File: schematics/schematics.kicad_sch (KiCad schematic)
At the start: 28 parts, among them SW1 RESET, U1 STM32F103VBT6, U2 AMS1117-3.3, Y1 16Mhz

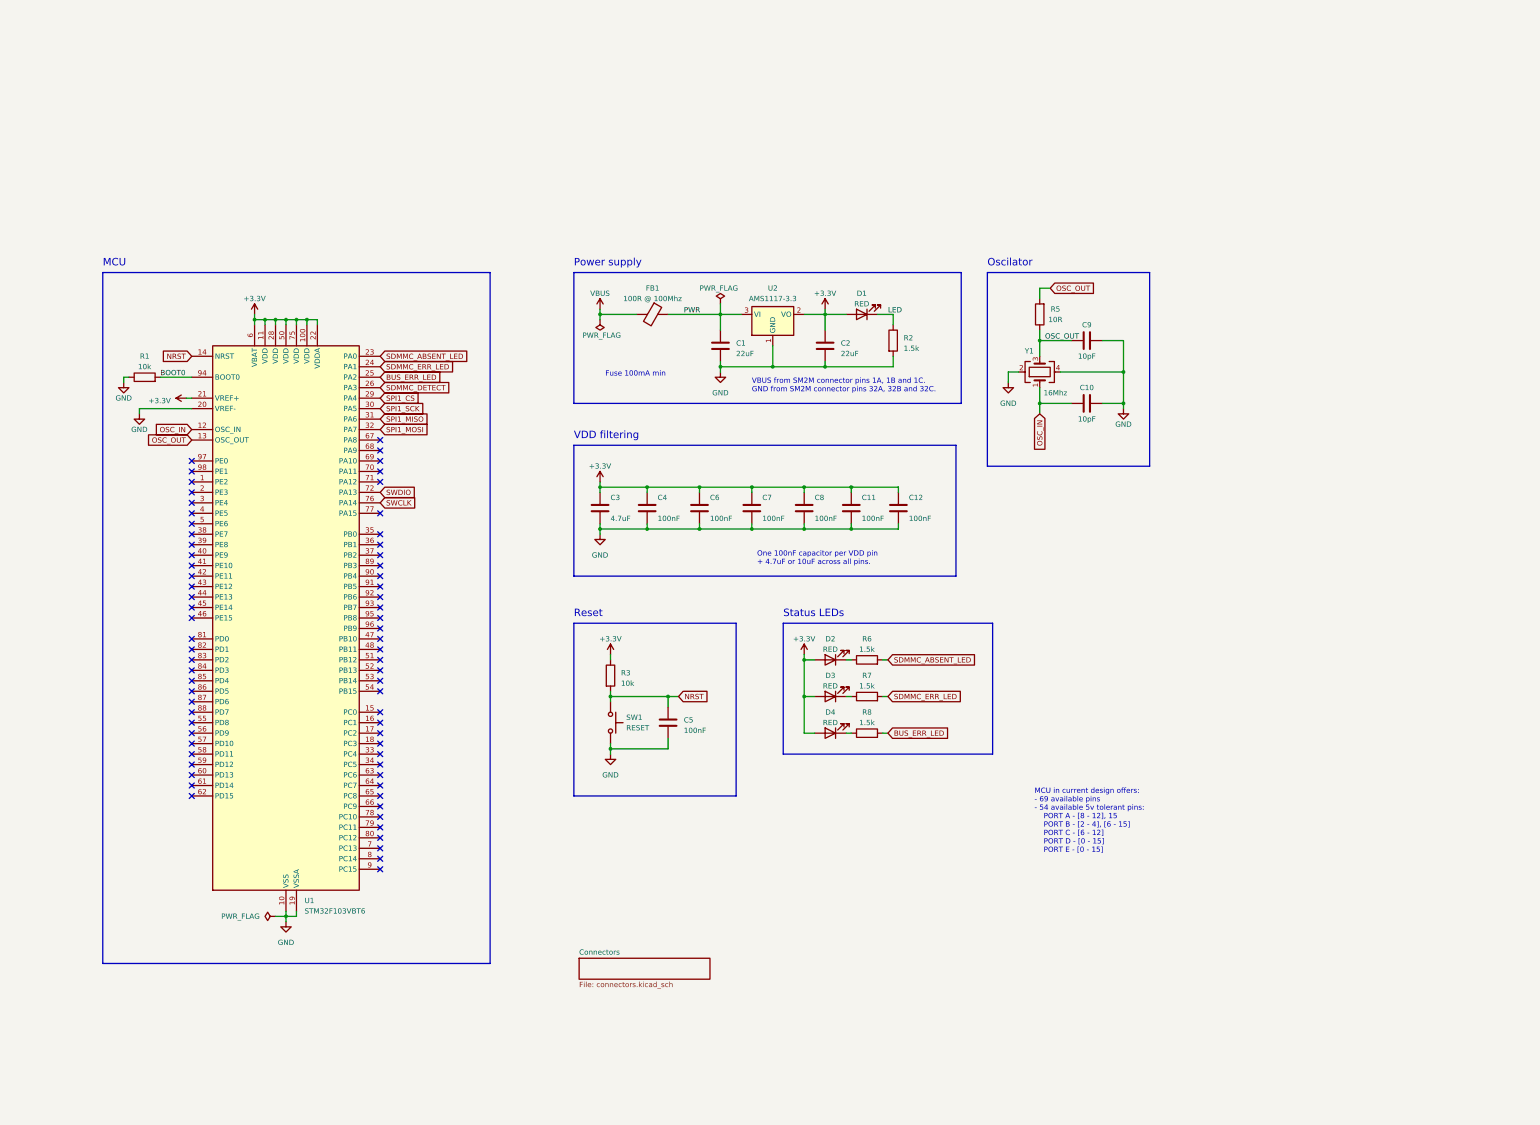
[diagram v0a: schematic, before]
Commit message: Update the board schematics
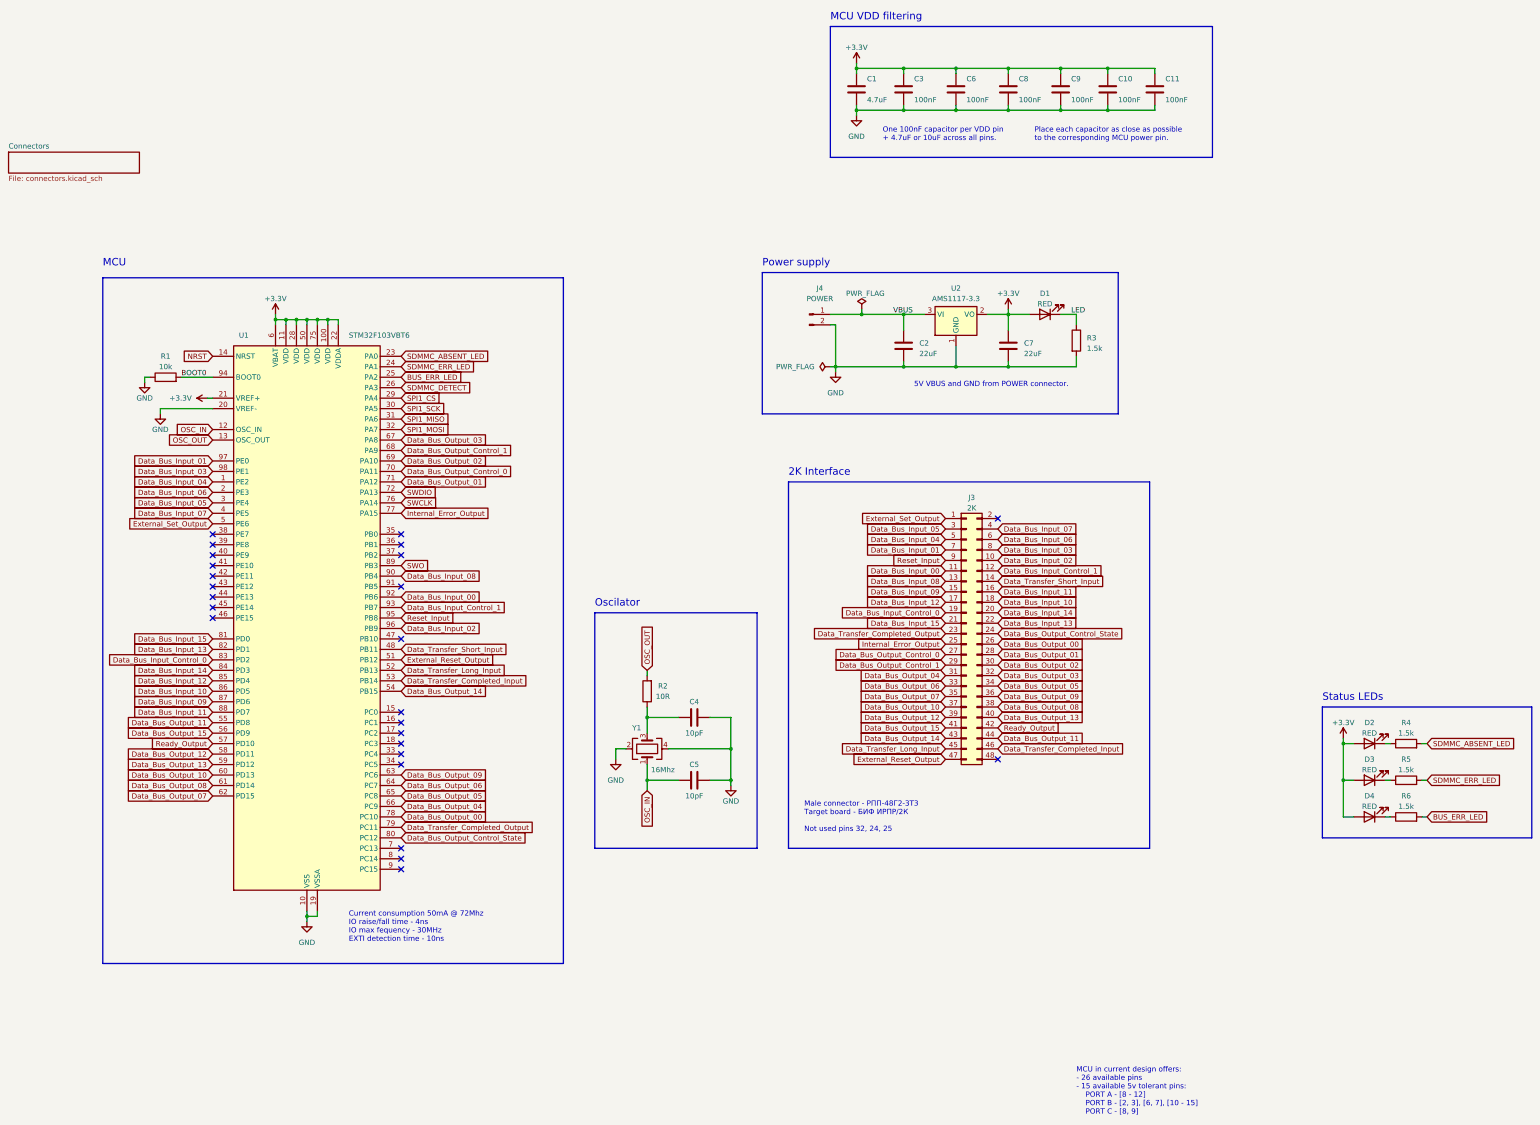
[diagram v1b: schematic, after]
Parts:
- removed C5: 100nF, Capacitor_SMD:C_0603_1608Metric, symbol Device:C
- removed FB1: 100R @ 100Mhz, Inductor_SMD:L_0603_1608Metric, symbol Device:FerriteBead
- removed R3: 10k, Resistor_SMD:R_0603_1608Metric, symbol Device:R
- removed SW1: RESET, Custom:SW_Push_SMD_4x4x1.5, symbol Switch:SW_Push
- added J3: 2K, Custom:RPP_48G2_3T3_Male, symbol Connector_Generic:Conn_02x24_Odd_Even
- added J4: POWER, Connector_JST:JST_EH_B2B-EH-A_1x02_P2.50mm_Vertical, symbol Connector:Conn_01x02_Pin
- renumbered C3 to C1, C11 to C10, C12 to C11, C1 to C2, C4 to C3, C9 to C4, C10 to C5, C2 to C7, C7 to C8, C8 to C9, R5 to R2, R2 to R3, R6 to R4, R7 to R5, R8 to R6
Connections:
- net PWR is gone; now on net VBUS: C2.1, U2.3 (VI)
- net GND: now also J4.2 (Pin_2)
- net OSC_OUT: no longer C4.1, R2.1, Y1.3
- net VBUS: now also J4.1 (Pin_1)
- net Data_Bus_Input_04: now reaches U1.1 (PE2)
- net Data_Bus_Input_04: now also J3.5 (Pin_5)
- net Data_Bus_Input_06: now reaches U1.2 (PE3)
- net Data_Bus_Input_06: now also J3.6 (Pin_6)
- net Data_Bus_Input_05: now reaches U1.3 (PE4)
- net Data_Bus_Input_05: now also J3.3 (Pin_3)
- net Data_Bus_Input_07: now reaches U1.4 (PE5)
- net Data_Bus_Input_07: now also J3.4 (Pin_4)
- net Data_Transfer_Short_Input: now reaches U1.48 (PB11)
- net Data_Transfer_Short_Input: now also J3.14 (Pin_14)
- net External_Set_Output: now reaches U1.5 (PE6)
- net External_Set_Output: now also J3.1 (Pin_1)
- net External_Reset_Output: now reaches U1.51 (PB12)
- net External_Reset_Output: now also J3.47 (Pin_47)
- net Data_Transfer_Long_Input: now reaches U1.52 (PB13)
- net Data_Transfer_Long_Input: now also J3.45 (Pin_45)
- net Data_Transfer_Completed_Input: now reaches U1.53 (PB14)
- net Data_Transfer_Completed_Input: now also J3.46 (Pin_46)
- net Data_Bus_Output_14: now reaches U1.54 (PB15)
- net Data_Bus_Output_14: now also J3.43 (Pin_43)
- net Data_Bus_Output_11: now reaches U1.55 (PD8)
- net Data_Bus_Output_11: now also J3.44 (Pin_44)
- net Data_Bus_Output_15: now reaches U1.56 (PD9)
- net Data_Bus_Output_15: now also J3.41 (Pin_41)
- net Ready_Output: now reaches U1.57 (PD10)
- net Ready_Output: now also J3.42 (Pin_42)
- net Data_Bus_Output_12: now reaches U1.58 (PD11)
- net Data_Bus_Output_12: now also J3.39 (Pin_39)
- net Data_Bus_Output_13: now reaches U1.59 (PD12)
- net Data_Bus_Output_13: now also J3.40 (Pin_40)
- net Data_Bus_Output_10: now reaches U1.60 (PD13)
- net Data_Bus_Output_10: now also J3.37 (Pin_37)
- net Data_Bus_Output_08: now reaches U1.61 (PD14)
- net Data_Bus_Output_08: now also J3.38 (Pin_38)
- net Data_Bus_Output_07: now reaches U1.62 (PD15)
- net Data_Bus_Output_07: now also J3.35 (Pin_35)
- net Data_Bus_Output_09: now reaches U1.63 (PC6)
- net Data_Bus_Output_09: now also J3.36 (Pin_36)
- net Data_Bus_Output_06: now reaches U1.64 (PC7)
- net Data_Bus_Output_06: now also J3.33 (Pin_33)
- net Data_Bus_Output_05: now reaches U1.65 (PC8)
- net Data_Bus_Output_05: now also J3.34 (Pin_34)
- net Data_Bus_Output_04: now reaches U1.66 (PC9)
- net Data_Bus_Output_04: now also J3.31 (Pin_31)
- net Data_Bus_Output_03: now reaches U1.67 (PA8)
- net Data_Bus_Output_03: now also J3.32 (Pin_32)
- net Data_Bus_Output_Control_1: now reaches U1.68 (PA9)
- net Data_Bus_Output_Control_1: now also J3.29 (Pin_29)
- net Data_Bus_Output_02: now reaches U1.69 (PA10)
- net Data_Bus_Output_02: now also J3.30 (Pin_30)
- net Data_Bus_Output_Control_0: now reaches U1.70 (PA11)
- net Data_Bus_Output_Control_0: now also J3.27 (Pin_27)
- net Data_Bus_Output_01: now reaches U1.71 (PA12)
- net Data_Bus_Output_01: now also J3.28 (Pin_28)
- net Internal_Error_Output: now reaches U1.77 (PA15)
- net Internal_Error_Output: now also J3.25 (Pin_25)
- net Data_Bus_Output_00: now reaches U1.78 (PC10)
- net Data_Bus_Output_00: now also J3.26 (Pin_26)
- net Data_Transfer_Completed_Output: now reaches U1.79 (PC11)
- net Data_Transfer_Completed_Output: now also J3.23 (Pin_23)
- net Data_Bus_Output_Control_State: now reaches U1.80 (PC12)
- net Data_Bus_Output_Control_State: now also J3.24 (Pin_24)
- net Data_Bus_Input_15: now reaches U1.81 (PD0)
- net Data_Bus_Input_15: now also J3.21 (Pin_21)
- net Data_Bus_Input_13: now reaches U1.82 (PD1)
- net Data_Bus_Input_13: now also J3.22 (Pin_22)
- net Data_Bus_Input_Control_0: now reaches U1.83 (PD2)
- net Data_Bus_Input_Control_0: now also J3.19 (Pin_19)
- net Data_Bus_Input_14: now reaches U1.84 (PD3)
- net Data_Bus_Input_14: now also J3.20 (Pin_20)
- net Data_Bus_Input_12: now reaches U1.85 (PD4)
- net Data_Bus_Input_12: now also J3.17 (Pin_17)
- net Data_Bus_Input_10: now reaches U1.86 (PD5)
- net Data_Bus_Input_10: now also J3.18 (Pin_18)
- net Data_Bus_Input_09: now reaches U1.87 (PD6)
- net Data_Bus_Input_09: now also J3.15 (Pin_15)
- net Data_Bus_Input_11: now reaches U1.88 (PD7)
- net Data_Bus_Input_11: now also J3.16 (Pin_16)
- net SWO: now reaches U1.89 (PB3)
- net Data_Bus_Input_08: now reaches U1.90 (PB4)
- net Data_Bus_Input_08: now also J3.13 (Pin_13)
- net Data_Bus_Input_00: now reaches U1.92 (PB6)
- net Data_Bus_Input_00: now also J3.11 (Pin_11)
- net Data_Bus_Input_Control_1: now reaches U1.93 (PB7)
- net Data_Bus_Input_Control_1: now also J3.12 (Pin_12)
- net Reset_Input: now reaches U1.95 (PB8)
- net Reset_Input: now also J3.9 (Pin_9)
- net Data_Bus_Input_02: now reaches U1.96 (PB9)
- net Data_Bus_Input_02: now also J3.10 (Pin_10)
- net Data_Bus_Input_01: now reaches U1.97 (PE0)
- net Data_Bus_Input_01: now also J3.7 (Pin_7)
- net Data_Bus_Input_03: now reaches U1.98 (PE1)
- net Data_Bus_Input_03: now also J3.8 (Pin_8)
- new net: C4.1, R2.1, Y1.3
- no-connect marks 70 -> 25
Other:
- note added: "2K Interface"
- note added: "5V VBUS and GND from POWER connector."
- note added: "Current consumption 50mA @ 72Mhz IO raise/fall time - 4ns IO max fequency - 30MHz EXTI detection time - 10ns"
- note added: "MCU VDD filtering"
- note added: "MCU in current design offers: - 26 available pins - 15 available 5v tolerant pins: PORT A - [8 - 12] PORT B - [2, 3], [6, 7], [10 - 15] PORT C - [8, 9]"
- note added: "Male connector - РПП-48Г2-3Т3 Target board - БИФ ИРПР/2К Not used pins 32, 24, 25"
- note added: "Place each capacitor as close as possible to the corresponding MCU power pin."
- note removed: "Fuse 100mA min"
- note removed: "MCU in current design offers: - 69 available pins - 54 available 5v tolerant pins: PORT A - [8 - 12], 15 PORT B - [2 - 4], [6 - 15] PORT C - [6 - 12] PORT D - [0 - 15] PORT E - [0 - 15]"
- note removed: "Reset"
- note removed: "VBUS from SM2M connector pins 1A, 1B and 1C. GND from SM2M connector pins 32A, 32B and 32C."
- note removed: "VDD filtering"
- moved on the sheet: C1, C10, C11, C2, C3, C4, C5, C6, C7, C8, C9, D1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
